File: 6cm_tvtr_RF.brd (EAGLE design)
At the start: 102.3 x 101.3 mm, 19 parts

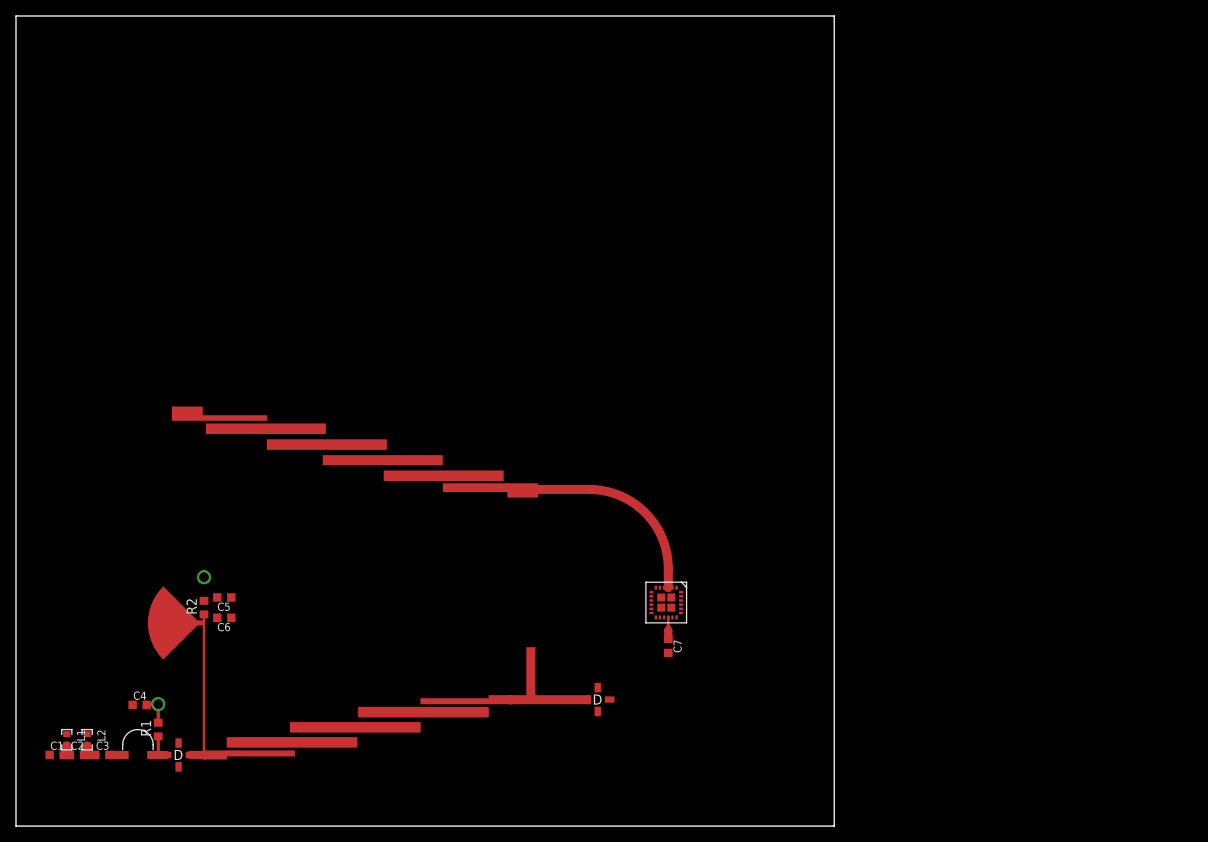
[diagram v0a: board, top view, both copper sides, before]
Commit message: layout with GAL1+ etc
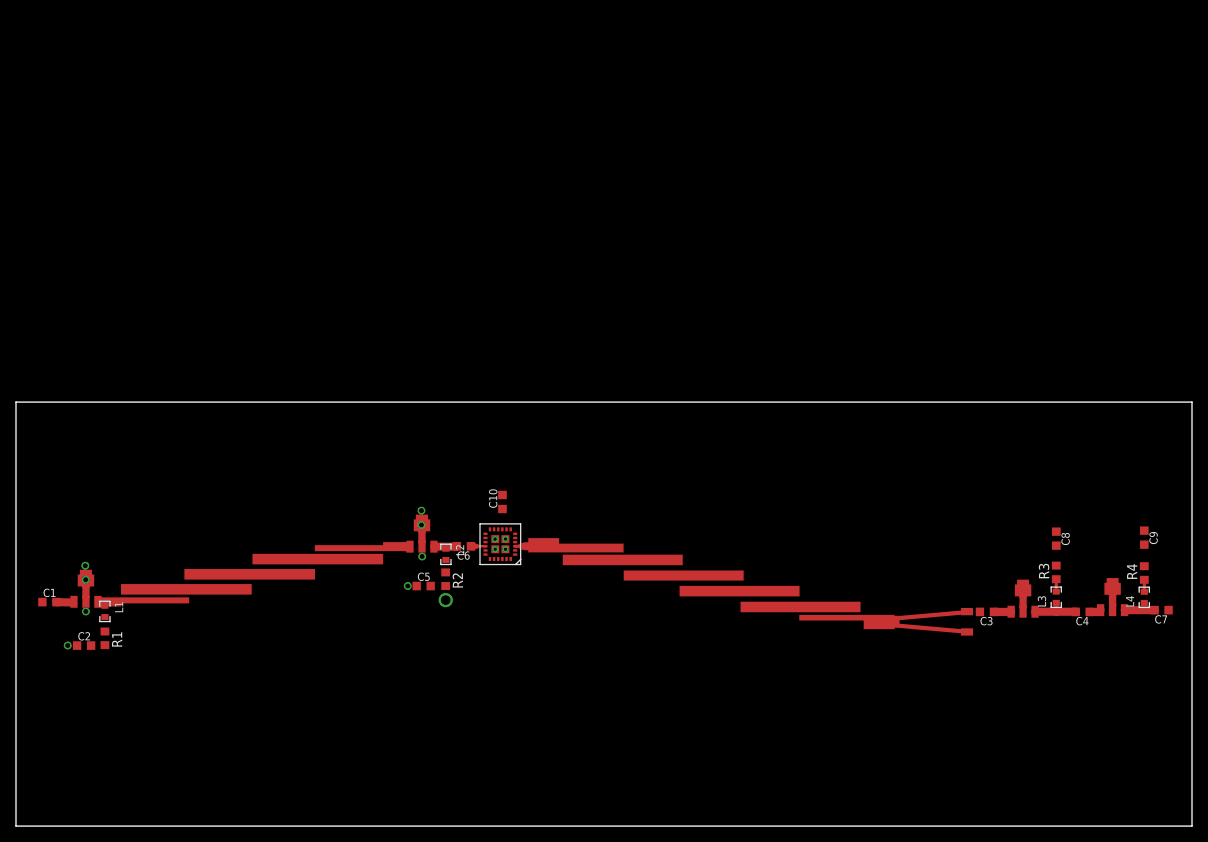
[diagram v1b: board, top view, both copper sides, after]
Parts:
- added C10, C8, C9: (no value), rcl:C0603K
- added L3, L4: 0603, inductors:0603
- added R3, R4: (no value), resistor:R0603
- U$1: value CE3512K2 -> GALI39+; device RF:CEL_FET -> RF:DF782
- U$2: value CE3512K2 -> GALI1+; device RF:CEL_FET -> RF:DF782
- U$3: value HAIRPIN -> GALI39+; device RF:HAIRPIN -> RF:DF782
- U$4: value 57_FLAKE -> GALI1+; device RF:FLAKE_576 -> RF:DF782
- U$7: value Q1_INPUT -> 576_WILK; device microstrip:Q1_INPUT -> RF:576_WILK
- moved C4 118.5 mm to (133.3, 26.8), turned to 180 degrees
- moved U$4 114.2 mm to (137.1, 27.0), turned to 0 degrees
- moved U$3 112.1 mm to (125.9, 26.8)
- moved C3 112.0 mm to (121.4, 26.8), turned to 180 degrees
- moved C7 61.8 mm to (143.2, 27.0), turned to 180 degrees
- moved L2 50.5 mm to (53.7, 34.0)
- moved U$7 49.1 mm to (110.0, 25.5)
- moved C6 31.3 mm to (56.0, 35.0)
- moved R2 30.4 mm to (53.7, 30.9), turned to 270 degrees
- moved U$2 29.1 mm to (50.7, 34.9)
- moved C5 25.0 mm to (51.0, 30.0), turned to 0 degrees
- moved U$5 23.2 mm to (45.9, 34.0)
- moved U$1 22.4 mm to (8.74, 28.0)
- moved U$8 22.0 mm to (60.5, 35.2), turned to 180 degrees
- moved C1 19.1 mm to (4.17, 28.0)
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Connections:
- removed net G1: C4.2, R1.2
- new net N$12: C3.1, U$3.P$1
- new net N$13: C4.2, L3.P$1, U$3.P$3
- new net N$14: C4.1, U$4.P$1
- new net N$15: C7.2, L4.P$1, U$4.P$3
- new net N$16: L3.P$2, R3.1
- new net N$17: L4.P$2, R4.1
- new net N$18: C10.1, U$8.P$9
- new net N$8: C1.1
- new net VCC: C2.2, R1.2
- net D1: now also C8.2, C9.2, R3.2, R4.2
- net GND: now also C2.1, C8.1, C9.1, U$1.P$2, U$1.P$4, U$1.P$5, U$1.P$6, U$1.P$7, U$1.P$8, U$2.P$2, U$2.P$4, U$2.P$5, U$2.P$6, U$2.P$7, U$2.P$8, U$3.P$2, U$3.P$4, U$3.P$5, U$3.P$6, U$3.P$7, U$3.P$8, U$4.P$2, U$4.P$4, U$4.P$5, U$4.P$6, U$4.P$7, U$4.P$8; no longer C4.1, C6.1, L1.P$1, L2.P$1, U$1.S1, U$1.S2, U$2.S1, U$2.S2
- net N$1: now also U$1.P$1; no longer C2.1, L1.P$2
- net N$10: now also C3.2, U$7.P$2; no longer U$2.D
- net N$2: now also R2.1; no longer C2.2, C3.1
- net N$3: now also C6.2, L2.P$1, U$2.P$3; no longer C3.2, U$3.P$1
- net N$4: now also L1.P$2; no longer U$1.G, U$3.P$2
- net N$5: now also L1.P$1, U$1.P$3; no longer C6.2, R2.1, U$1.D, U$4.P$1
- net N$6: now also U$2.P$1; no longer U$7.N
- net N$7: now also U$6.P$2, U$7.P$1; no longer U$2.G, U$7.OUT
- net N$9: now also C6.1; no longer C7.1
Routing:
- net N$11: track 23.3 -> 2.16 mm
- net N$5: track 18.8 -> 0.00 mm
- net N$13: track 0.00 -> 6.23 mm
- net N$4: track 4.01 -> 0.00 mm
- net G1: track 3.78 -> 0.00 mm, vias 1 -> 0
- net N$15: track 0.00 -> 3.75 mm
- net N$2: track 2.63 -> 0.00 mm
- net N$12: track 0.00 -> 2.17 mm
- net N$16: track 0.00 -> 1.56 mm
- net N$17: track 0.00 -> 1.50 mm
- net N$14: track 0.00 -> 1.46 mm
- net N$3: track 1.67 -> 2.89 mm
- net N$9: track 2.69 -> 1.75 mm
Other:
- board size 102.3 x 101.3 mm -> 147 x 53 mm
